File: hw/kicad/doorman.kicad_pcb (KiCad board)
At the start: 2 copper layers, 28 x 80 mm, 20 parts, among them J1 RDet, J2 Lock, J3 PWR, K1 S1A05, Q1 BC337, U1 WeMos_D1_mini, U2 PC817

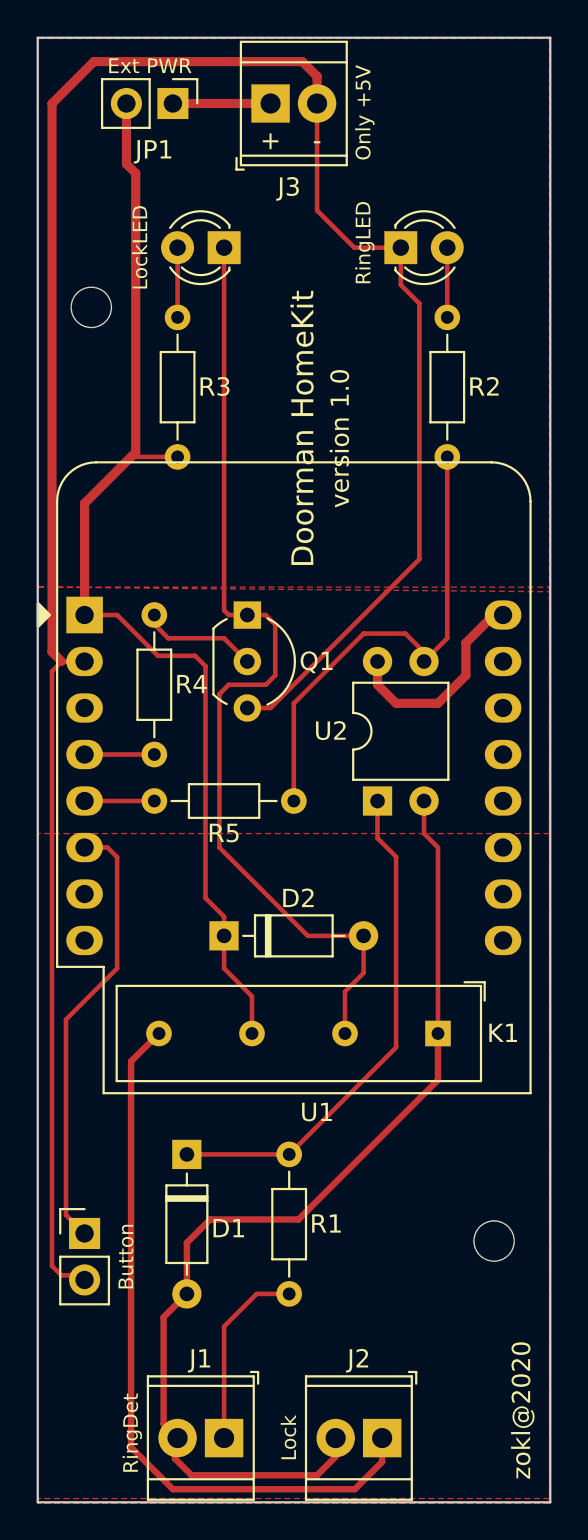
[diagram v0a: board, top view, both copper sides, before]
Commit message: Final PCB.
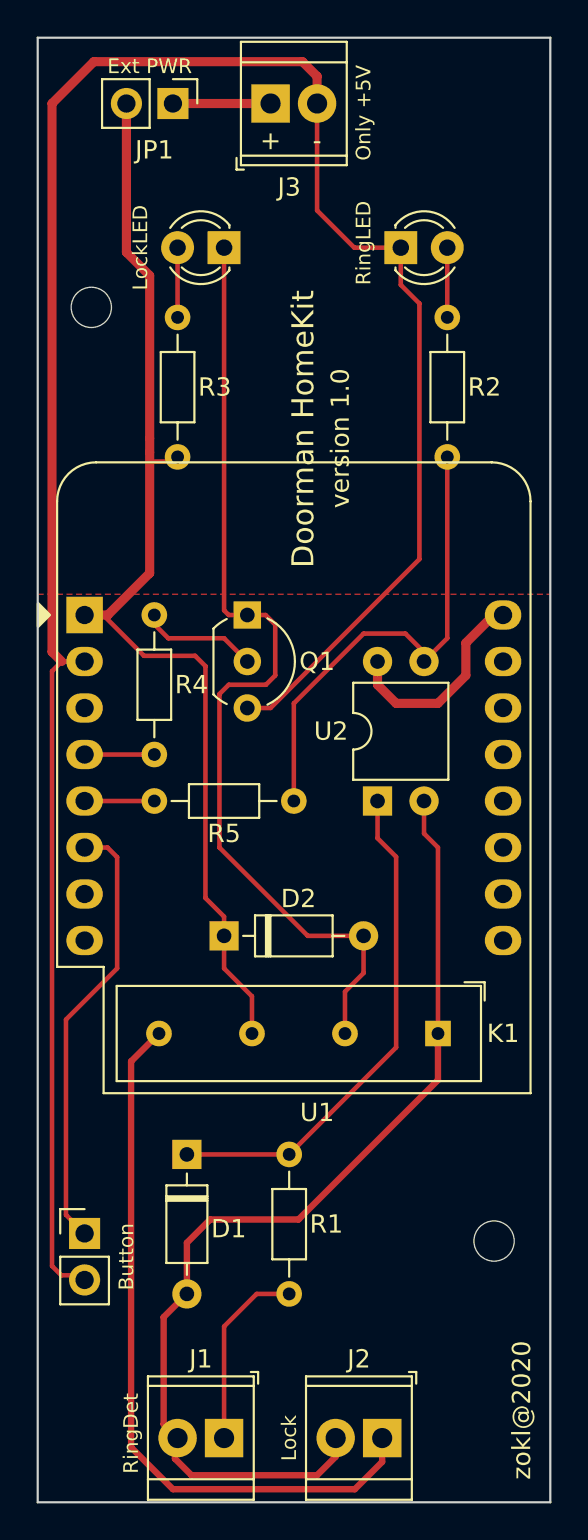
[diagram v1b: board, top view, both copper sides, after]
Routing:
- net +5V: track 60.7 -> 61.7 mm
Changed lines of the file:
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@@
-(kicad_pcb (version 20171130) (host pcbnew "(5.1.5-0-10_14)")
+(kicad_pcb (version 20171130) (host pcbnew 5.1.5-52549c5~84~ubuntu18.04.1)
   (general
     (thickness 1.6)
     (drawings 19)
-    (tracks 112)
+    (tracks 115)
     (zones 0)
     (modules 20)
@@
     (last_trace_width 0.25)
     (trace_clearance 0.2)
-    (zone_clearance 0.508)
+    (zone_clearance 0.48)
     (zone_45_only no)
     (trace_min 0.2)
@@
     (solder_mask_min_width 0.25)
     (aux_axis_origin 0 0)
+    (grid_origin 101.072 51.27)
     (visible_elements FFFFFF7F)
     (pcbplotparams
@@
   (segment (start 111.252 100.33) (end 111.252 102.108) (width 0.25) (layer F.Cu) (net 4))
   (segment (start 111.252 102.108) (end 112.776 103.632) (width 0.25) (layer F.Cu) (net 4))
-  (segment (start 106.172 74.168) (end 108.712 74.168) (width 0.25) (layer F.Cu) (net 4))
-  (segment (start 103.632 76.708) (end 106.172 74.168) (width 0.5) (layer F.Cu) (net 4))
-  (segment (start 103.632 82.804) (end 103.632 76.708) (width 0.5) (layer F.Cu) (net 4))
-  (segment (start 106.426 73.914) (end 106.172 74.168) (width 0.5) (layer F.Cu) (net 4))
-  (segment (start 106.426 58.674) (end 106.426 73.914) (width 0.5) (layer F.Cu) (net 4))
-  (segment (start 105.918 58.166) (end 106.426 58.674) (width 0.5) (layer F.Cu) (net 4))
-  (segment (start 105.918 54.864) (end 105.918 58.166) (width 0.5) (layer F.Cu) (net 4))
+  (segment (start 107.188 64.262) (end 107.188 73.152) (width 0.5) (layer F.Cu) (net 4))
+  (segment (start 105.918 62.992) (end 107.188 64.262) (width 0.5) (layer F.Cu) (net 4))
+  (segment (start 105.918 54.864) (end 105.918 62.992) (width 0.5) (layer F.Cu) (net 4))
+  (segment (start 107.188 73.914) (end 107.188 73.152) (width 0.5) (layer F.Cu) (net 4))
+  (segment (start 108.458 74.422) (end 108.712 74.168) (width 0.25) (layer F.Cu) (net 4))
+  (segment (start 107.188 74.422) (end 108.458 74.422) (width 0.25) (layer F.Cu) (net 4))
+  (segment (start 107.188 73.914) (end 107.188 74.422) (width 0.25) (layer F.Cu) (net 4))
+  (segment (start 107.188 80.518) (end 107.188 73.914) (width 0.5) (layer F.Cu) (net 4))
+  (segment (start 104.902 82.804) (end 107.188 80.518) (width 0.5) (layer F.Cu) (net 4))
+  (segment (start 103.632 82.804) (end 104.902 82.804) (width 0.5) (layer F.Cu) (net 4))
   (segment (start 111.252 99.28) (end 111.252 100.33) (width 0.25) (layer F.Cu) (net 4))
+  (segment (start 110.236 98.264) (end 111.252 99.28) (width 0.25) (layer F.Cu) (net 4))
+  (segment (start 104.648 82.804) (end 106.87601 85.03201) (width 0.25) (layer F.Cu) (net 4))
   (segment (start 110.236 85.598) (end 110.236 98.264) (width 0.25) (layer F.Cu) (net 4))
-  (segment (start 110.236 98.264) (end 111.252 99.28) (width 0.25) (layer F.Cu) (net 4))
-  (segment (start 103.632 82.804) (end 105.41 82.804) (width 0.25) (layer F.Cu) (net 4))
-  (segment (start 107.63801 85.03201) (end 109.67001 85.03201) (width 0.25) (layer F.Cu) (net 4))
-  (segment (start 105.41 82.804) (end 107.63801 85.03201) (width 0.25) (layer F.Cu) (net 4))
+  (segment (start 106.87601 85.03201) (end 109.67001 85.03201) (width 0.25) (layer F.Cu) (net 4))
   (segment (start 109.67001 85.03201) (end 110.236 85.598) (width 0.25) (layer F.Cu) (net 4))
+  (segment (start 103.632 82.804) (end 104.648 82.804) (width 0.25) (layer F.Cu) (net 4))
   (segment (start 113.03 119.888) (end 114.808 119.888) (width 0.25) (layer F.Cu) (net 5))
   (segment (start 111.252 121.666) (end 113.03 119.888) (width 0.25) (layer F.Cu) (net 5))
@@
   (segment (start 126.492 82.804) (end 125.984 82.804) (width 0.5) (layer F.Cu) (net 16))
   (zone (net 7) (net_name GND) (layer F.Cu) (hatch edge 0.508)
-    (connect_pads (clearance 0.508))
+    (connect_pads (clearance 0.48))
     (min_thickness 0.254)
-    (fill (arc_segments 32) (thermal_gap 0.508) (thermal_bridge_width 0.508))
+    (fill yes (arc_segments 32) (thermal_gap 0.48) (thermal_bridge_width 0.48))
     (polygon
       (pts
-        (xy 129.032 131.064) (xy 101.092 131.064) (xy 101.092 51.308) (xy 129.032 51.308)
+        (xy 129.072 131.27) (xy 101.072 131.27) (xy 101.072 81.67) (xy 129.072 81.67)
       )
     )
-  )
-  (zone (net 7) (net_name GND) (layer F.Cu) (hatch edge 0.508)
-    (connect_pads (clearance 0.508))
-    (min_thickness 0.254)
-    (fill (arc_segments 32) (thermal_gap 0.508) (thermal_bridge_width 0.508))
-    (polygon
-      (pts
-        (xy 129.032 131.318) (xy 101.092 131.318) (xy 101.092 51.308) (xy 129.032 51.308)
-      )
-    )
-  )
-  (zone (net 7) (net_name GND) (layer F.Cu) (hatch edge 0.508)
-    (connect_pads (clearance 0.508))
-    (min_thickness 0.254)
-    (fill (arc_segments 32) (thermal_gap 0.508) (thermal_bridge_width 0.508))
-    (polygon
-      (pts
-        (xy 129.032 131.318) (xy 101.092 131.318) (xy 101.092 51.308) (xy 129.032 51.308)
-      )
-    )
-  )
-  (zone (net 7) (net_name GND) (layer F.Cu) (hatch edge 0.508)
-    (connect_pads (clearance 0.508))
-    (min_thickness 0.254)
-    (fill (arc_segments 32) (thermal_gap 0.508) (thermal_bridge_width 0.508))
-    (polygon
-      (pts
-        (xy 129.032 94.742) (xy 101.092 94.742) (xy 101.092 81.28) (xy 129.032 81.28)
-      )
-    )
-  )
-  (zone (net 7) (net_name GND) (layer F.Cu) (hatch edge 0.508)
-    (connect_pads (clearance 0.508))
-    (min_thickness 0.254)
-    (fill yes (arc_segments 32) (thermal_gap 0.508) (thermal_bridge_width 0.508))
-    (polygon
-      (pts
-        (xy 129.032 81.534) (xy 129.032 131.318) (xy 101.092 131.318) (xy 101.092 81.28)
-      )
-    )
